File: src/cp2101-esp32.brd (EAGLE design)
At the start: 45 x 18.6 mm, 24 parts, among them IC1 LM1117MPX-3.3, J1 USB4105_REVA, T1 BC847, T2 BC847, U1 CP2102-GM

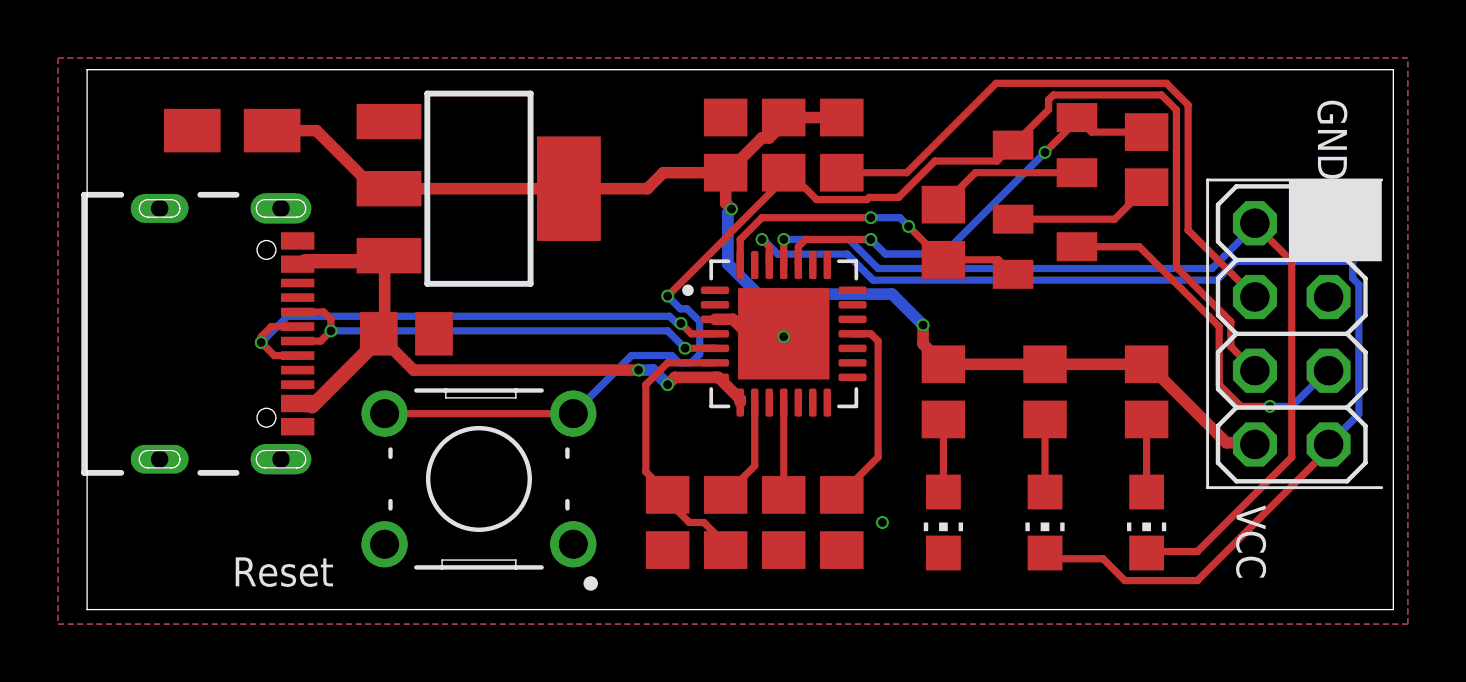
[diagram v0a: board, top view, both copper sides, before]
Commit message: .
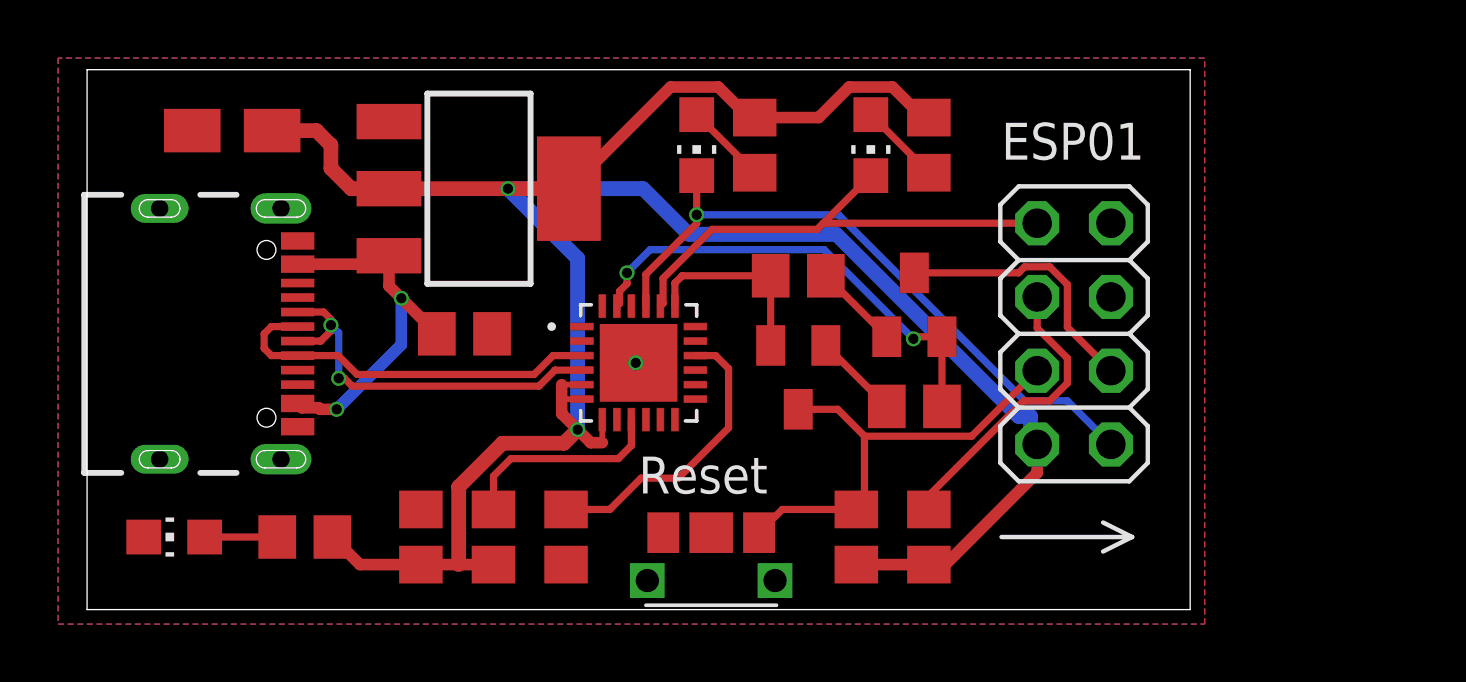
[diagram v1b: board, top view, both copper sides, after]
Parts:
- removed C3: 10u, rcl:C0805
- removed R1, R7: 4.7K, rcl:R0805
- removed S1: B3F-1000, B3F-1000:SW_B3F-1000
- added R8: 10K, rcl:R0805
- added U$1: SWITCH2X4-MICRO, SMD Tact:2X4-MICRO
- U1: value CP2102-GM -> CP2104-F03-GM; device CP2102-GM:QFN50P500X500X100-29N -> CP2104:QFN50P400X400X80-25N
- moved LED1 26.5 mm to (3.00, 2.50), turned to 90 degrees
- moved R4 22.6 mm to (7.50, 2.50), turned to 0 degrees
- moved LED2 17.7 mm to (21.0, 16.0)
- moved C8 17.1 mm to (11.5, 2.50)
- moved LED3 16.1 mm to (27.0, 16.0)
- moved R9 13.8 mm to (29.0, 2.50), turned to 270 degrees
- moved R10 13.7 mm to (26.5, 2.50), turned to 270 degrees
- moved R5 13.1 mm to (23.0, 16.0)
- moved R3 12.6 mm to (24.5, 11.5), turned to 0 degrees
- moved T1 11.7 mm to (24.5, 8.00), turned to 180 degrees
- moved R6 11.3 mm to (29.0, 16.0)
- moved C1 9.51 mm to (16.5, 2.50)
- moved JP2 7.50 mm to (34.0, 9.50)
- moved R2 6.08 mm to (28.5, 7.00), turned to 180 degrees
- moved U1 5.10 mm to (19.0, 8.50)
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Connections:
- removed net !RST: R1.1, U1.9
- removed net !SUSPEND: R7.2, U1.11
- removed net VDD: C3.1, R1.2, U1.6
- new net N$7: C1.1, U1.16
- net +3V3: now also R8.2, U1.5, U1.6, U1.7
- net D+: now also U1.3; no longer U1.4
- net D-: now also U1.4; no longer U1.5
- net DTR: now also U1.23; no longer U1.28
- net GND: now also U$1.P$5, U1.2, U1.25; no longer C3.2, R7.1, S1.1, S1.2, U1.29, U1.3
- net N$1: now also R8.1, U1.9; no longer C1.1, U1.18
- net RST: now also U$1.P$4; no longer S1.3, S1.4
- net RTS: now also U1.19; no longer U1.24
- net RXD: now also U1.20; no longer U1.25
- net TXD: now also U1.21; no longer U1.26
- net VBUS: no longer U1.7, U1.8
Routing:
- net +3V3: track 46.1 -> 85.3 mm
- net RST: track 46.3 -> 15.9 mm, vias 1 -> 0
- net TXD: track 41.3 -> 22.8 mm
- net RXD: track 33.2 -> 17.0 mm, vias 1 -> 0
- net VBUS: track 23.7 -> 12.8 mm
- net CH_PD: track 21.1 -> 10.3 mm
- net N$7: track 0.00 -> 10.1 mm
- net VDD: track 9.82 -> 0.00 mm
- net RTS: track 15.1 -> 6.60 mm, vias 2 -> 0
- net D+: track 19.3 -> 13.3 mm, vias 2 -> 0
- net DTR: track 11.5 -> 16.2 mm
- net !RST: track 3.59 -> 0.00 mm
- net IO0: track 12.6 -> 9.20 mm, vias 1 -> 0
- net !SUSPEND: track 3.18 -> 0.00 mm
- net D-: track 16.4 -> 13.6 mm
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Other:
- board size 45 x 18.6 mm -> 38 x 18.6 mm
- board text added: "3.3V"
- board text added: "CH_PD"
- board text added: "ESP01"
- board text added: "IO0"
- board text added: "IO2"
- board text added: "RST"
- board text added: "RXD"
- board text added: "TXD"
- board text added: "USB - UART"
- board text added: "https://ovcharov.me"
- board text removed: "VCC"
